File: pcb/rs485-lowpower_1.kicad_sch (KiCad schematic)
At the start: 16 parts, among them U4 MAX487

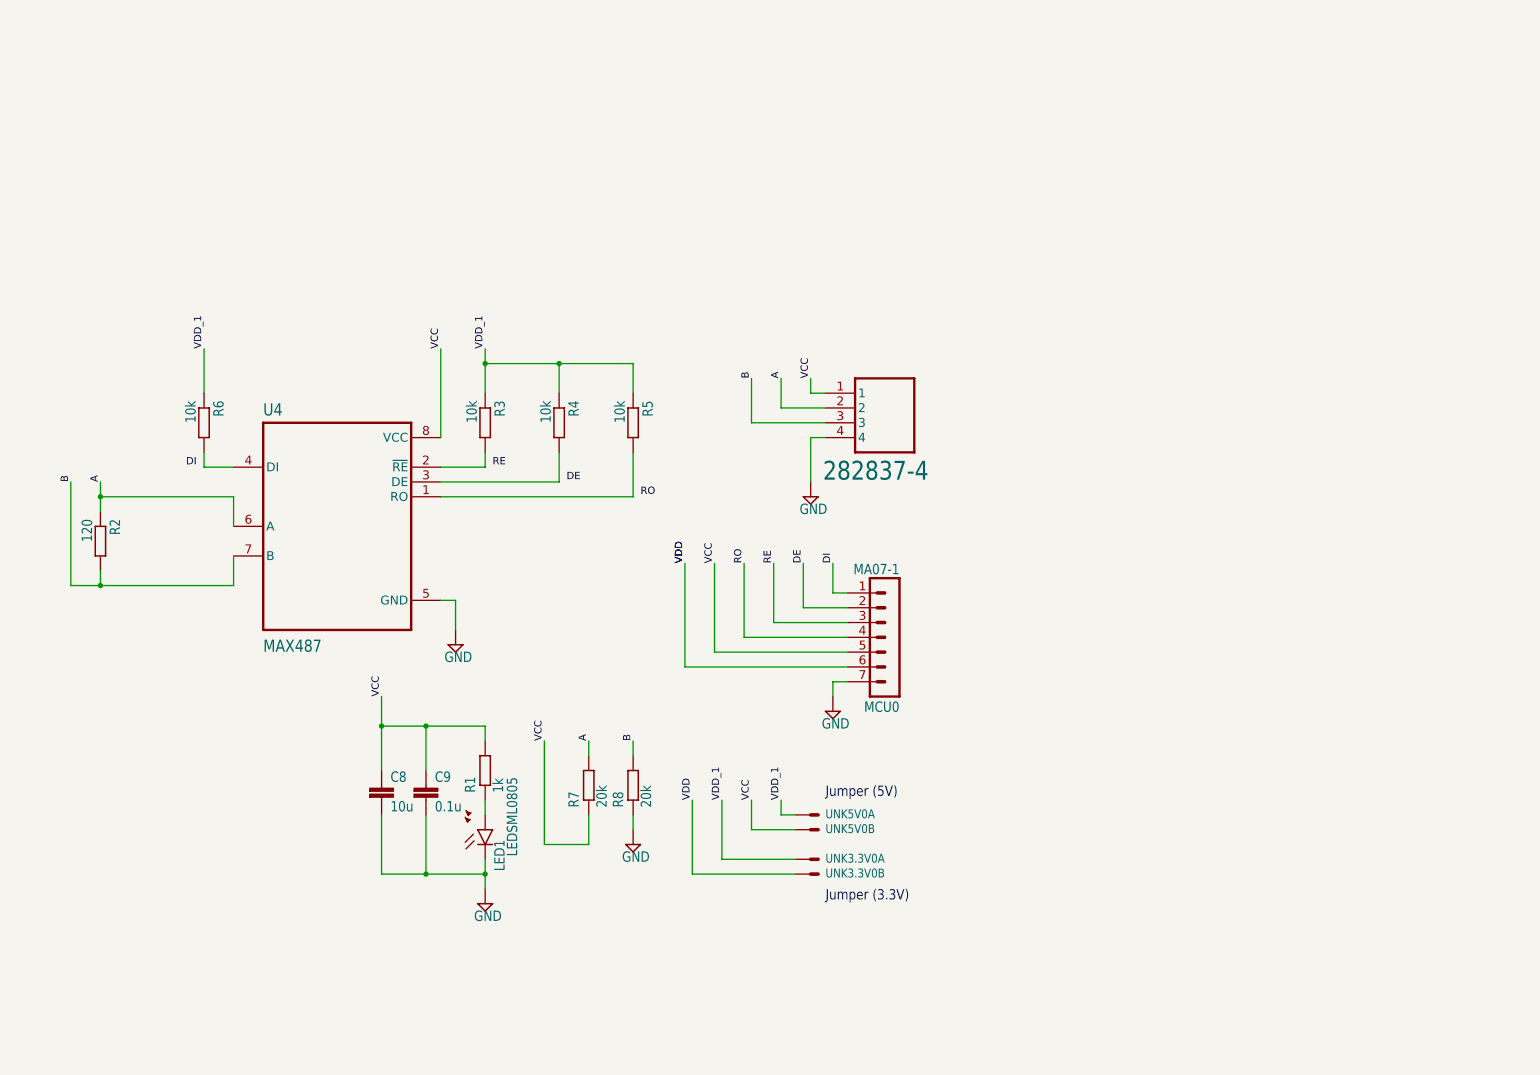
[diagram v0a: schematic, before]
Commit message: reupload pcb file
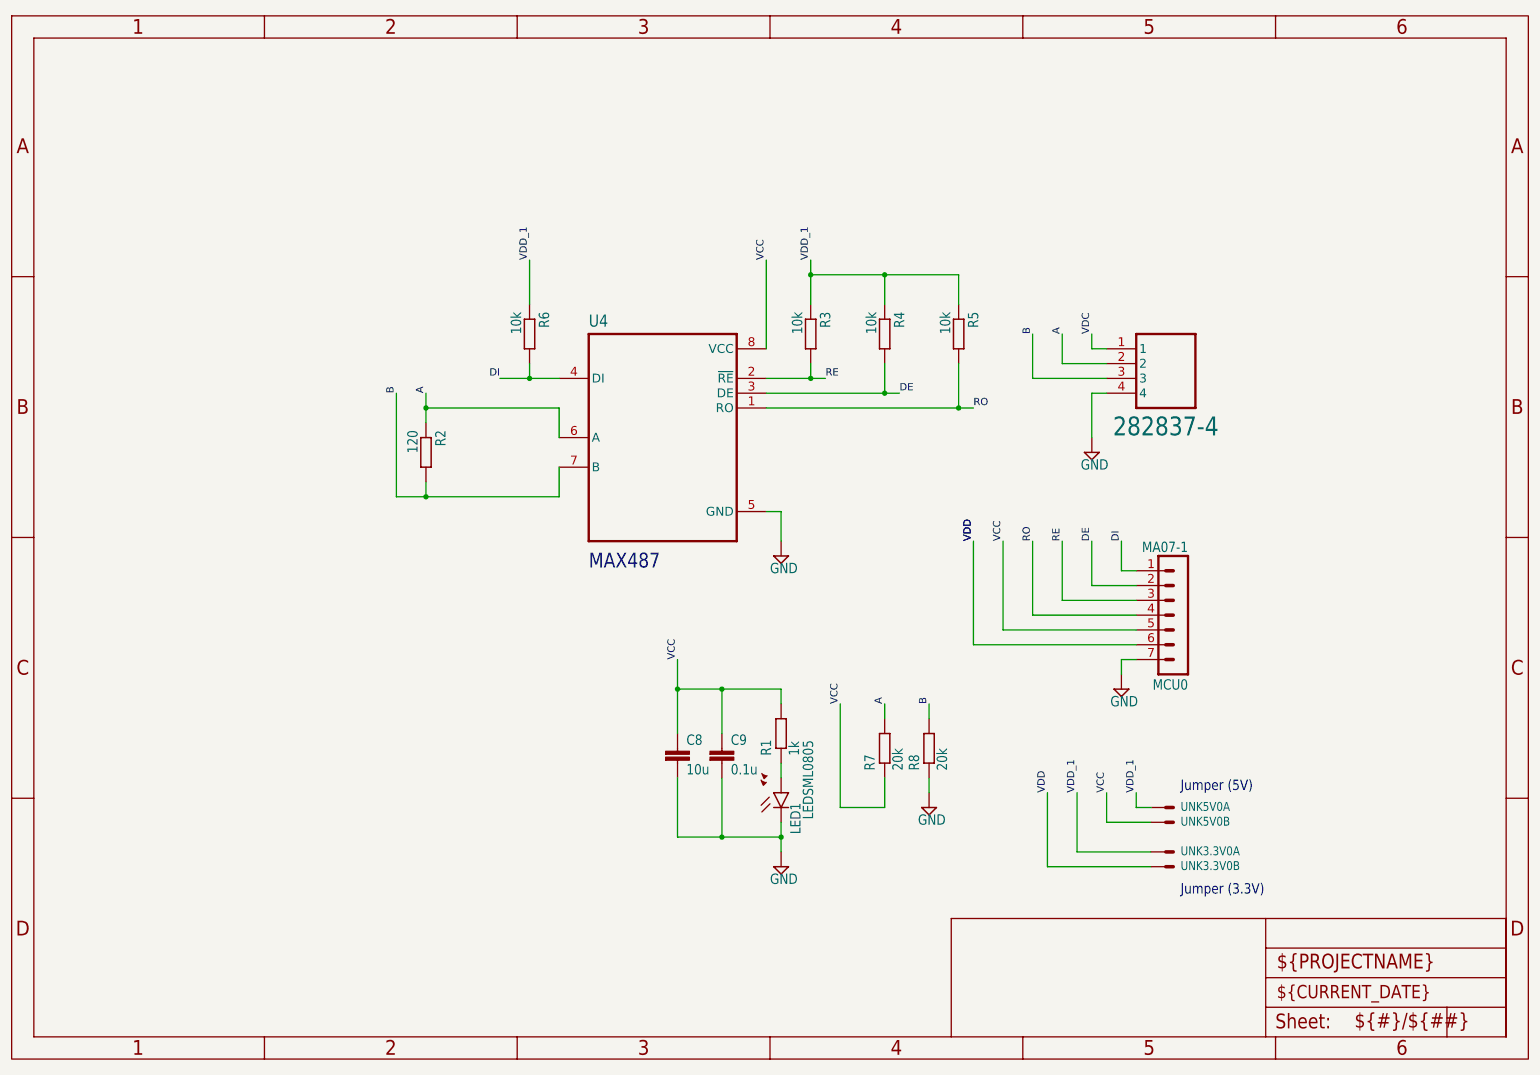
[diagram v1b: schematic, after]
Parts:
- U4: value MAX487 -> MAX485CSA+T
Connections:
- net DE: now also R4.2, U4.3 (DE)
- net DI: now also R6.2, U4.4 (DI)
- net RE: now also R3.2, U4.2 (~{RE})
- net RO: now also R5.2, U4.1 (RO)
- net VCC: no longer RS485-UGMLPV1.0.1
- new net VDC: RS485-UGMLPV1.0.1
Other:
- note added: "MAX487"
